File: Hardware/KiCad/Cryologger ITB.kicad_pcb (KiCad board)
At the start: 2 copper layers, 133 x 63 mm, 18 parts, among them J1 Screw_Terminal_01x02, U1 Adafruit_LSM303AGR, U2 Pololu_D36V6x, U6 Adafruit_BME280, U8 RockBLOCK_Footprint, U9 Pololu_D36V6x

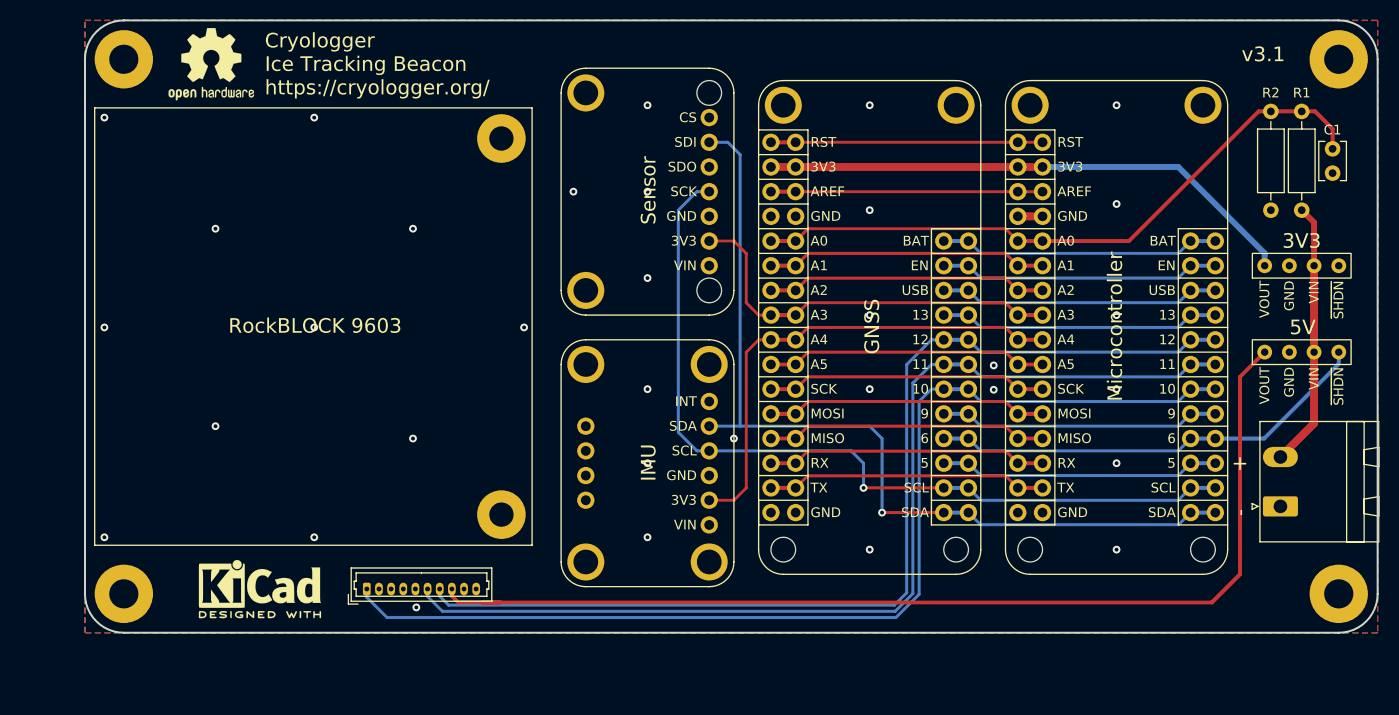
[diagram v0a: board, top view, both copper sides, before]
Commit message: Minor updates to PCB design
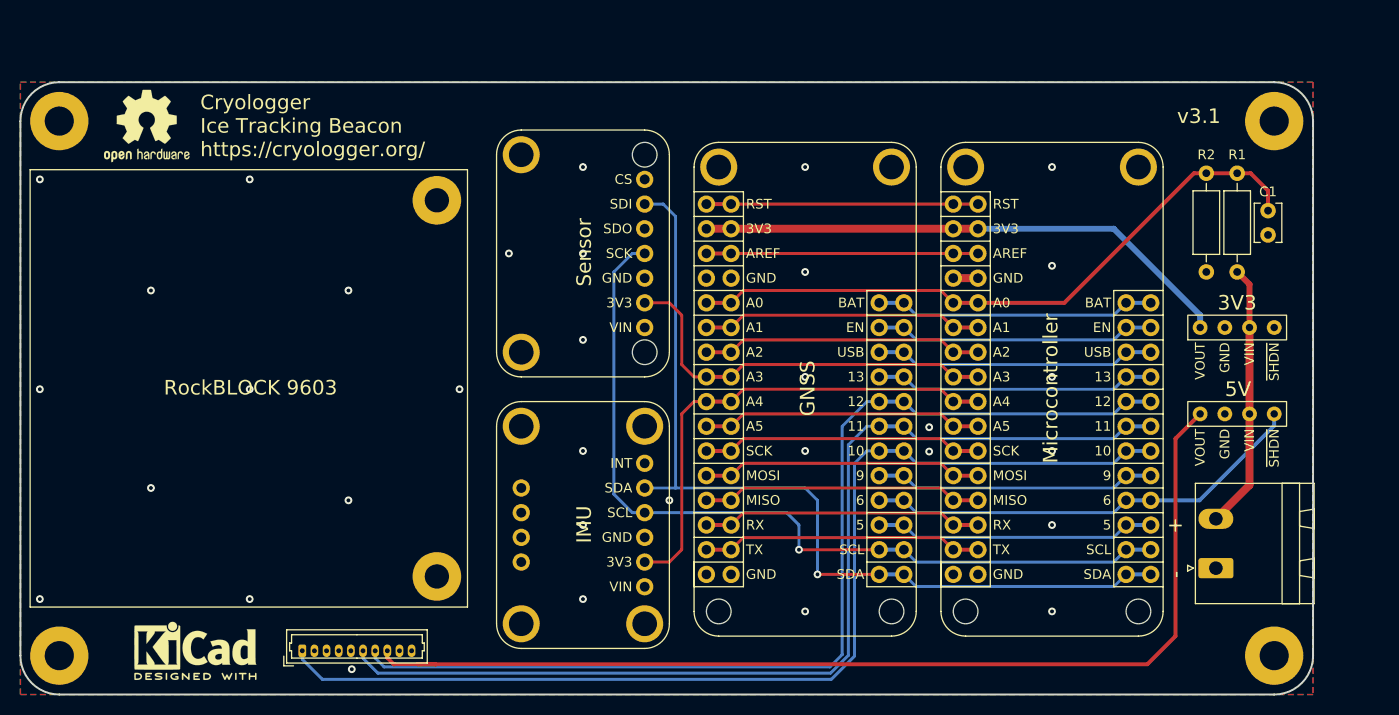
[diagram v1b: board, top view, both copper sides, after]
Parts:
- moved H1 9.19 mm to (80.4, 125.4)
- moved H2 9.19 mm to (80.4, 70.4)
- moved H3 9.19 mm to (205.4, 70.4)
- moved H4 9.19 mm to (205.4, 125.4)
- moved J1 9.19 mm to (199.4, 116.4)
- moved R2 9.19 mm to (198.4, 75.7)
- moved REF** 9.19 mm to (89.4, 70.9)
- moved REF** 9.19 mm to (94.4, 124.9)
- moved U1 9.19 mm to (134.2, 111.9)
- moved U3 9.19 mm to (105.4, 124.9)
- moved U8 9.19 mm to (99.9, 97.9)
- moved A2 9.19 mm to (157.1, 97.9)
- moved A3 9.19 mm to (182.5, 97.9)
- moved C1 9.19 mm to (204.7, 79.6)
- moved R1 9.19 mm to (201.5, 85.9)
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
